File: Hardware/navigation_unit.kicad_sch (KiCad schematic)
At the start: 43 parts, among them U4 STM32F405RGT6, U5 TDD01H0SB1R, U6 TDD01H0SB1R, Y1 25MHz

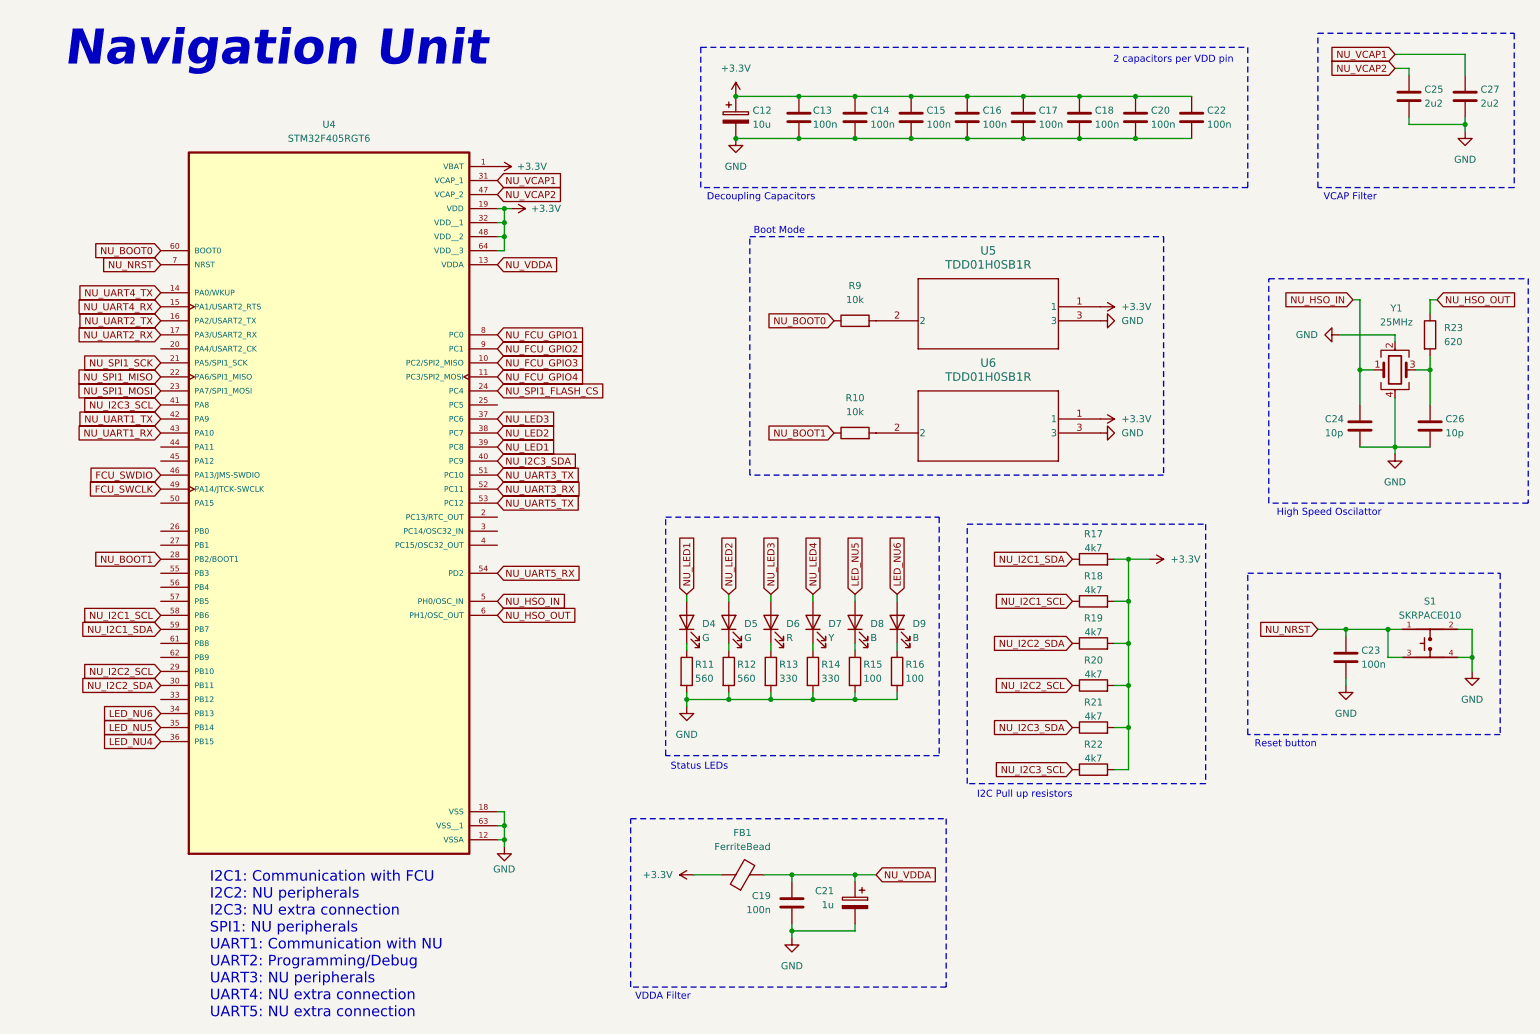
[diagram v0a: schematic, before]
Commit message: pin mess up win, starting over again
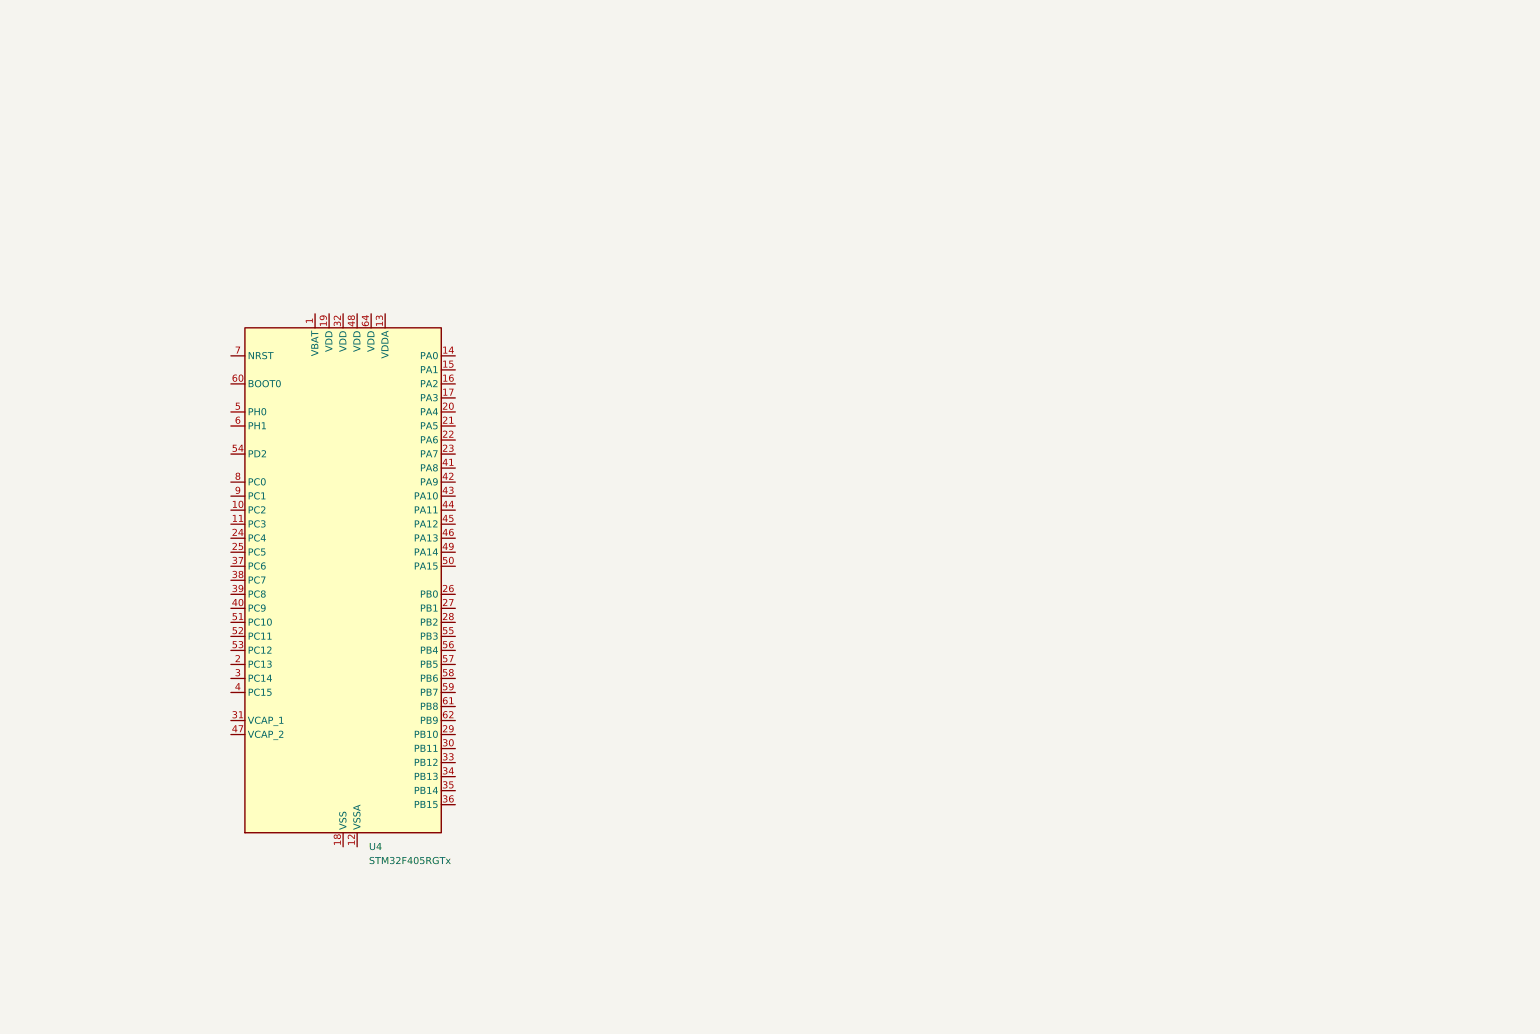
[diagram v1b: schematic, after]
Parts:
- removed C12: 10u, symbol Device:C_Polarized
- removed C13, C14, C15, C16, C17, C18, C19, C20, C22, C23: 100n, symbol Device:C
- removed C21: 1u, symbol Device:C_Polarized
- removed C24, C26: 10p, symbol Device:C
- removed C25, C27: 2u2, symbol Device:C
- removed D4, D5: G, symbol Device:LED
- removed D6: R, symbol Device:LED
- removed D7: Y, symbol Device:LED
- removed D8, D9: B, symbol Device:LED
- removed FB1: FerriteBead, symbol Device:FerriteBead
- removed R10, R9: 10k, symbol Device:R
- removed R11, R12: 560, symbol Device:R
- removed R13, R14: 330, symbol Device:R
- removed R15, R16: 100, symbol Device:R
- removed R17, R18, R19, R20, R21, R22: 4k7, symbol Device:R
- removed R23: 620, symbol Device:R
- removed S1: SKRPACE010, SKRPACE010:SW_SKRPACE010, symbol Aircraft_Components:SKRPACE010
- removed U4: STM32F405RGT6, STM32F405RGT6:QFP50P1200X1200X160-64N, symbol Aircraft_Components:STM32F405RGT6
- removed U5, U6: TDD01H0SB1R, SOT_TDDSB1R_CNK, symbol Aircraft_Components:TDD01H0SB1R
- removed Y1: 25MHz, symbol Device:Crystal_GND24
- added U4: STM32F405RGTx, Package_QFP:LQFP-64_10x10mm_P0.5mm, symbol MCU_ST_STM32F4:STM32F405RGTx
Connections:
- new net: U4.18 (VSS), U4.63 (VSS)
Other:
- note removed: "2 capacitors per VDD pin"
- note removed: "Boot Mode"
- note removed: "Decoupling Capacitors"
- note removed: "High Speed Oscilattor"
- note removed: "I2C Pull up resistors"
- note removed: "I2C1: Communication with FCU I2C2: NU peripherals I2C3: NU extra connection SPI1: NU peripherals UART1: Communication with NU UART2: Programming/Debug UART3: NU peripherals UART4: NU extra connection UART5: NU extra connection"
- note removed: "Navigation Unit"
- note removed: "Reset button"
- note removed: "Status LEDs"
- note removed: "VCAP Filter"
- note removed: "VDDA Filter"
